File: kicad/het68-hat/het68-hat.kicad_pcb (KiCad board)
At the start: 2 copper layers, 94 x 96 mm, 91 parts, among them J1 MIC1, J10 PWR, J11 PZ1, J12 PZ2, J13 PZ3, J14 PZ4, J17 UART, J2 MIC2, J3 MIC3, J4 MIC4, J5 MIC5, J6 MIC6, U1 Pico_Plus_2, U2 SN74LVC8T245, U3 SN74LVC8T245, U4 SN74LVC8T245, U5 AP2112K-1.8, U6 DRV8837C, U7 DPS310, U8 SHT40, U9 INA3221

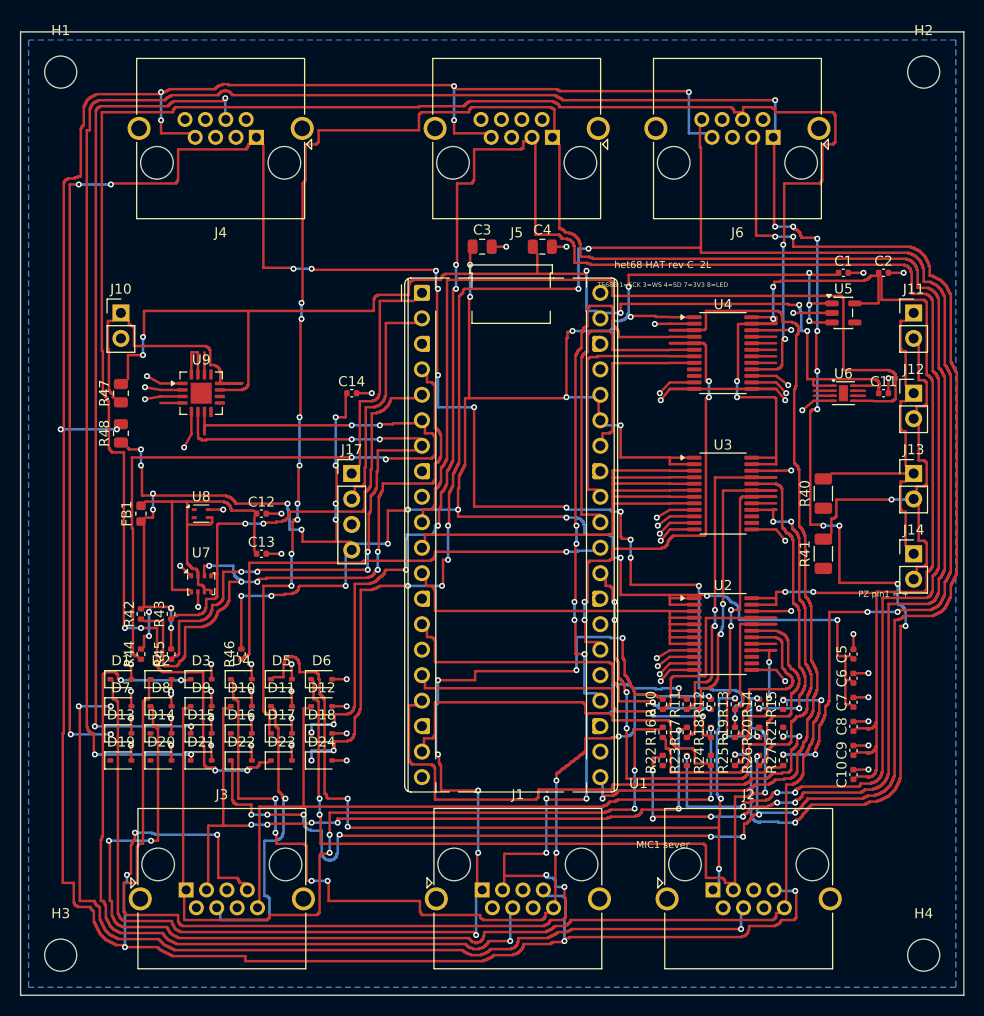
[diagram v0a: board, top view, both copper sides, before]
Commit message: Protect the CT secondary and ship clean power and satellite fab files.
Add burden, LC filter and crowbar on the power board, close DRC on power and satellite, and refresh the board previews for v1.10.0.

Co-authored-by: Cursor <cursoragent@cursor.com>
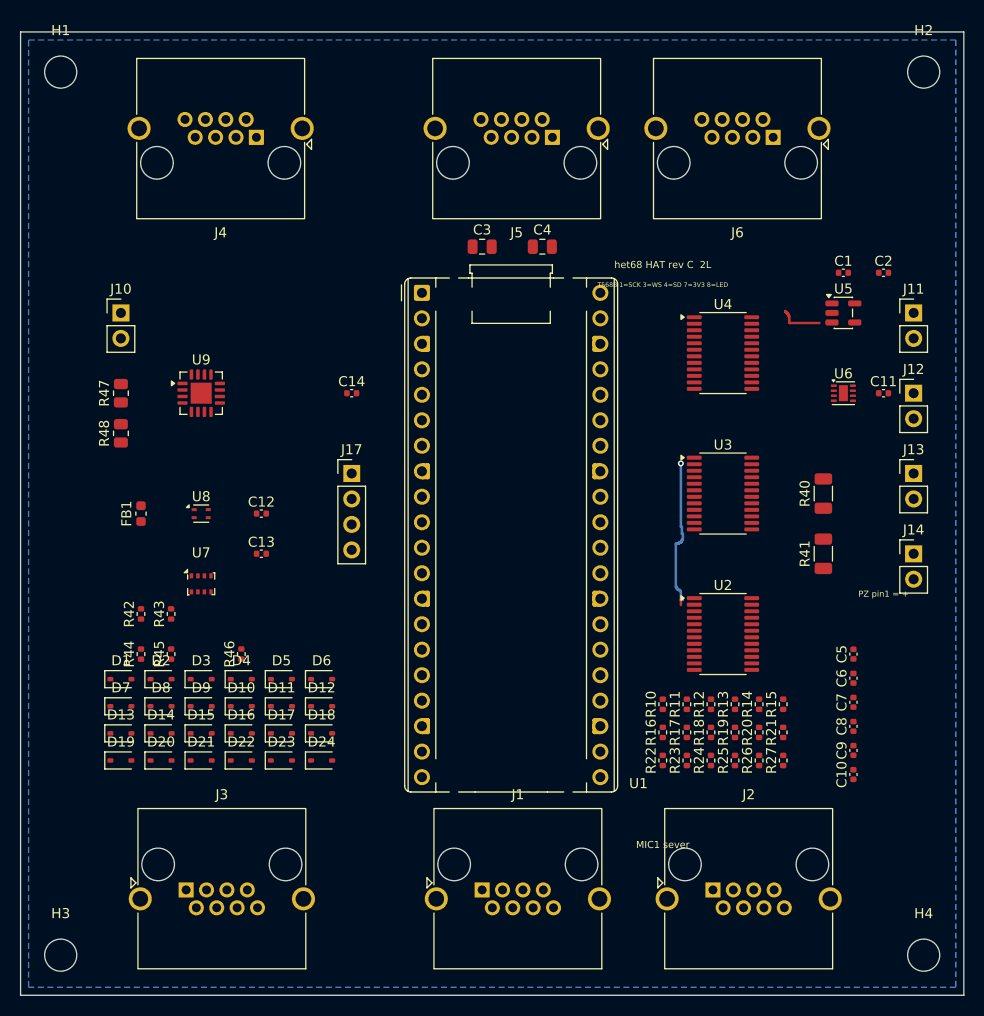
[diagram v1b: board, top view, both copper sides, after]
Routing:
- net +3V3_MIC: track 299.8 -> 0.00 mm, vias 13 -> 0
- net +3V3: track 295.4 -> 20.3 mm, vias 34 -> 1
- net SCK6: track 256.7 -> 0.00 mm, vias 15 -> 0
- net SCK5: track 236.5 -> 0.00 mm, vias 14 -> 0
- net WS5: track 217.5 -> 0.00 mm, vias 10 -> 0
- net LED6: track 194.9 -> 0.00 mm, vias 12 -> 0
- net SD6_18: track 194.3 -> 0.00 mm, vias 6 -> 0
- net SCK4: track 188.3 -> 0.00 mm, vias 16 -> 0
- net WS6: track 180.6 -> 0.00 mm, vias 11 -> 0
- net GND: track 168.7 -> 0.00 mm, vias 66 -> 0
- net +1V8: track 137.5 -> 0.00 mm, vias 6 -> 0
- net LED2: track 126.8 -> 0.00 mm, vias 4 -> 0
- net SCK1: track 123.3 -> 0.00 mm, vias 7 -> 0
- net WS1: track 122.5 -> 0.00 mm, vias 6 -> 0
- net VSYS: track 115.7 -> 0.00 mm, vias 6 -> 0
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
